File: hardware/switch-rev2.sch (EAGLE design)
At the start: 100 parts, among them IC1 KS8995MA, IC2 MEGA168-20AU, Y1 12MHz, Y2 25MHz

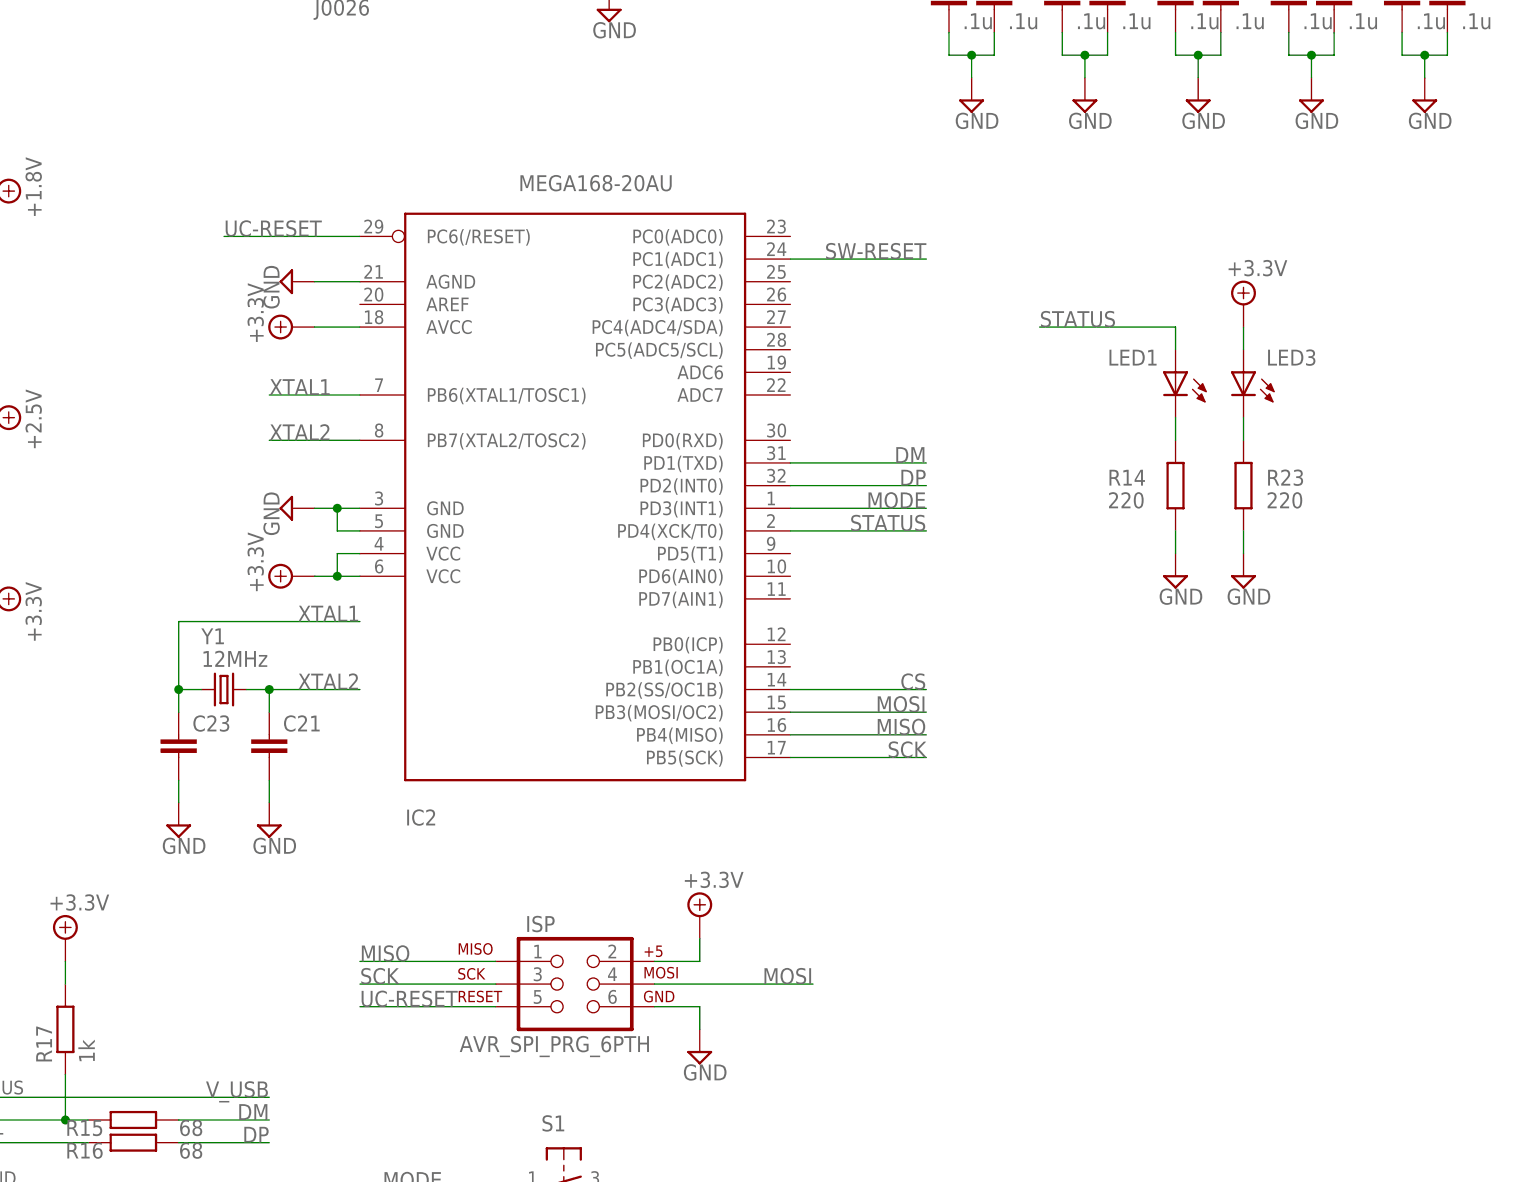
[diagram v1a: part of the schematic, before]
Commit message: hw: rev2: change atmega QFN package
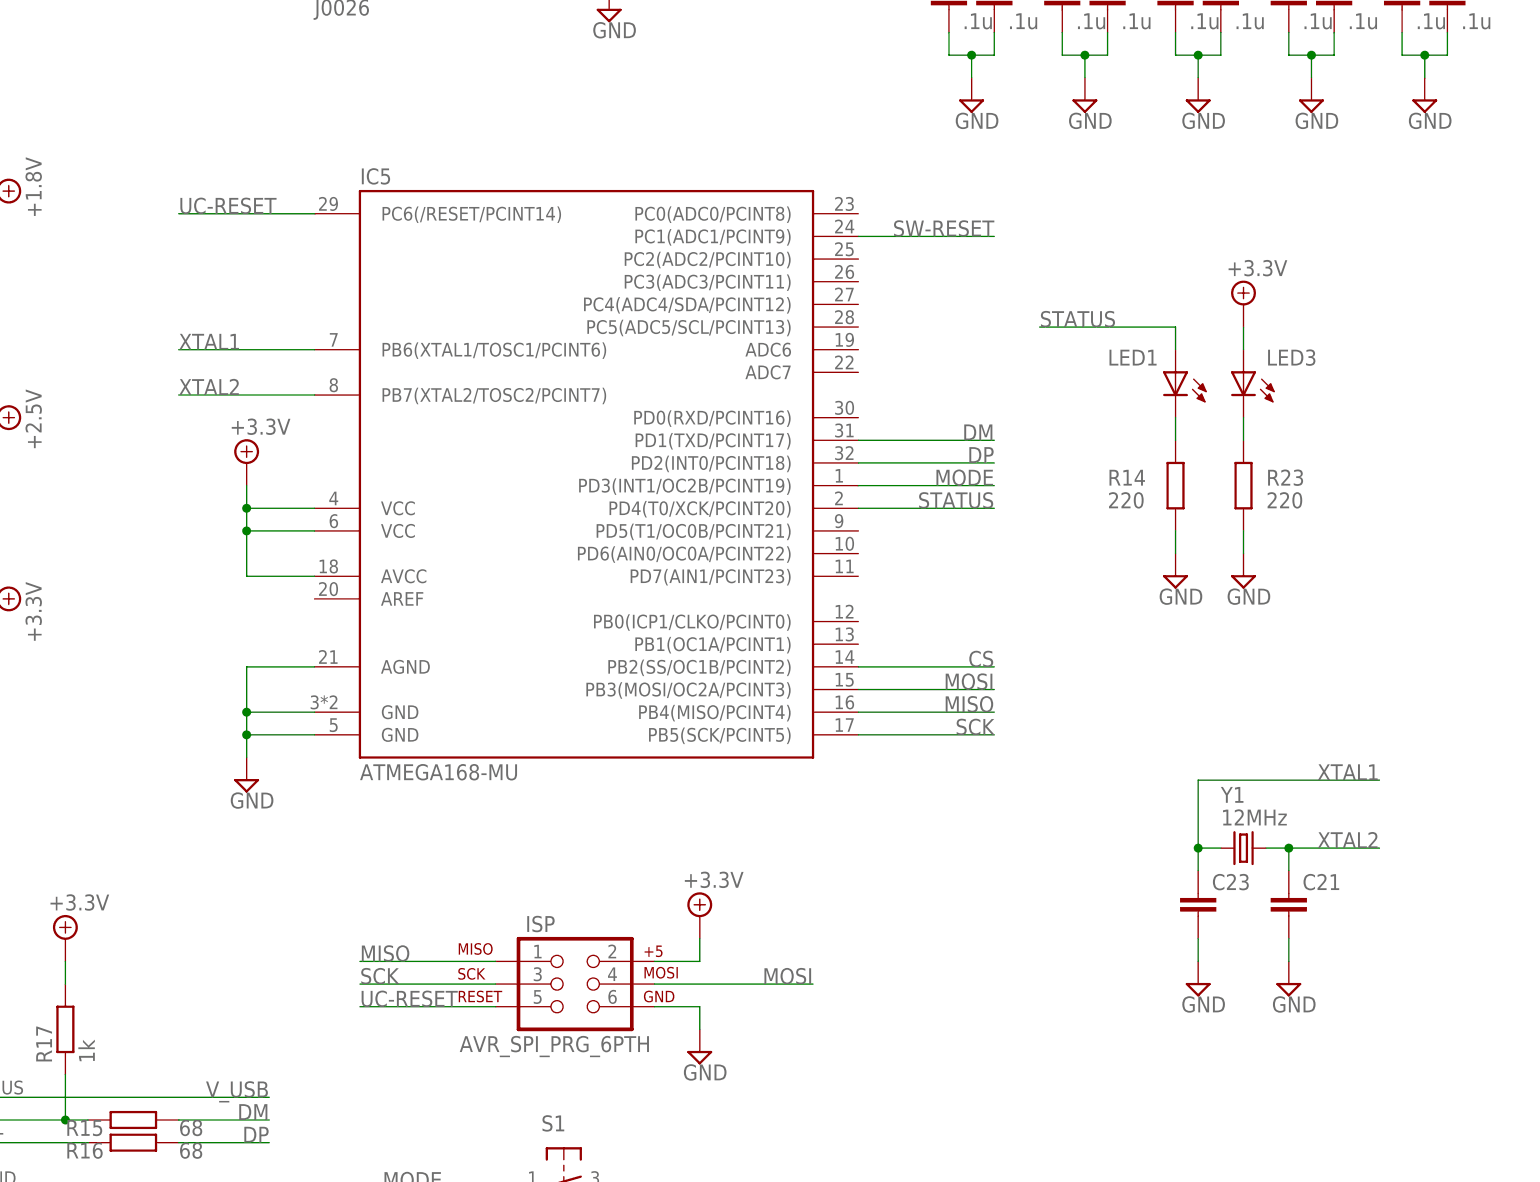
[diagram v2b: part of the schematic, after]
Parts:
- removed IC2: MEGA168-20AU, atmel:MEGA8-MI
- added IC5: ATMEGA168-MU, balto:ATMEGA168-MU
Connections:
- net +5V: now also IC5.AVCC, IC5.VCC@1, IC5.VCC@2; no longer IC2.AVCC, IC2.VCC@1, IC2.VCC@2
- net CS: now also IC5.PB2(SS/OC1B/PCINT2); no longer IC2.PB2(SS/OC1B)
- net DM: now also IC5.PD1(TXD/PCINT17); no longer IC2.PD1(TXD)
- net DP: now also IC5.PD2(INT0/PCINT18); no longer IC2.PD2(INT0)
- net GND: now also IC5.AGND, IC5.GND@1, IC5.GND@2; no longer IC2.AGND, IC2.GND@1, IC2.GND@2
- net MISO: now also IC5.PB4(MISO/PCINT4); no longer IC2.PB4(MISO)
- net MODE: now also IC5.PD3(INT1/OC2B/PCINT19); no longer IC2.PD3(INT1)
- net MOSI: now also IC5.PB3(MOSI/OC2A/PCINT3); no longer IC2.PB3(MOSI/OC2)
- net SCK: now also IC5.PB5(SCK/PCINT5); no longer IC2.PB5(SCK)
- net STATUS: now also IC5.PD4(T0/XCK/PCINT20); no longer IC2.PD4(XCK/T0)
- net SW-RESET: now also IC5.PC1(ADC1/PCINT9); no longer IC2.PC1(ADC1)
- net UC-RESET: now also IC5.PC6(/RESET/PCINT14); no longer IC2.PC6(/RESET)
- net XTAL1: now also IC5.PB6(XTAL1/TOSC1/PCINT6); no longer IC2.PB6(XTAL1/TOSC1)
- net XTAL2: now also IC5.PB7(XTAL2/TOSC2/PCINT7); no longer IC2.PB7(XTAL2/TOSC2)
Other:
- moved on the sheet: C21, C23, Y1
